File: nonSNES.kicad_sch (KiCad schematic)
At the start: 311 parts, among them J1 Jack-DC, P1 CASSETTE, P2 Conn_2Rows-11Pins, P3 Conn_01x02_Pin, Q10 C2412K, Q11 C2412K, Q12 C2412K, Q13 C2412K, Q14 C2412K, Q15 C2412K, Q16 C2412K, Q17 C2412K, Q18 C2412K, Q3 C2412K, Q4 C2412K, Q5 C2412K, Q6 C2412K, Q7 C2412K, Q8 C2412K, Q9 C2412K, SW1 RESET SW, T1 L_Coupled, U1 CPU, U10 LM324, U12 L7805, U13 S-SMP, U14 S-DSP, U15 MS62256CL-10FC, U16 MS62256CL-10FC, U17 uPD6376, U18 S-CLK, U2 PPU1, U3 PPU2, U4 MS62256CL-10FC, U5 MS62256CL-10FC, U6 WRAM, U7 S-ENC, U8 CIC, X1 17.734MHz, X2 24.576MHz

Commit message: fix errors
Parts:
- renumbered C20 to C12
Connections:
- net /IRQ: now also P5.26 (~{IRQ}), TP21.1
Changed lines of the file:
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@@
     )
   )
-  (global_label "{slash}IRQ" (shape input) (at 159.385 311.15 0) (fields_autoplaced)
+  (global_label "{slash}IRQ" (shape input) (at 158.75 311.15 0) (fields_autoplaced)
     (effects (font (size 1.27 1.27)) (justify left))
-    (property "Intersheetrefs" "${INTERSHEET_REFS}" (at 166.906 311.15 0)
+    (property "Intersheetrefs" "${INTERSHEET_REFS}" (at 166.271 311.15 0)
       (effects (font (size 1.27 1.27)) (justify left) hide)
     )
@@
   (symbol (lib_id "Device:C") (at 516.255 149.225 0) (unit 1)
     (in_bom yes) (on_board yes) (dnp no)
-    (property "Reference" "C20" (at 518.795 147.955 0)
+    (property "Reference" "C12" (at 518.795 147.955 0)
       (effects (font (size 1.27 1.27)) (justify left))
     )
@@
       (project "nonSNES"
         (path "/d1480d56-b791-43e1-bd4c-b0c74bb0533d"
-          (reference "C20") (unit 1)
+          (reference "C12") (unit 1)
         )
       )

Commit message: flip around most of the silkscreen on the bottom
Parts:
- renumbered C5 to C2, C2 to C5, C96 to C69, C69 to C96
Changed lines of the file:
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@@
   (symbol (lib_id "Device:C") (at 170.815 402.59 0) (mirror y) (unit 1)
     (in_bom no) (on_board yes) (dnp yes)
-    (property "Reference" "C96" (at 163.83 402.59 90)
+    (property "Reference" "C69" (at 163.83 402.59 90)
       (effects (font (size 1.27 1.27)))
     )
@@
       (project "nonSNES"
         (path "/d1480d56-b791-43e1-bd4c-b0c74bb0533d"
-          (reference "C96") (unit 1)
+          (reference "C69") (unit 1)
         )
       )
@@
   (symbol (lib_id "Device:C") (at 351.155 35.56 180) (unit 1)
     (in_bom yes) (on_board yes) (dnp no) (fields_autoplaced)
-    (property "Reference" "C69" (at 354.33 34.29 0)
+    (property "Reference" "C96" (at 354.33 34.29 0)
       (effects (font (size 1.27 1.27)) (justify right))
     )
@@
       (project "nonSNES"
         (path "/d1480d56-b791-43e1-bd4c-b0c74bb0533d"
-          (reference "C69") (unit 1)
+          (reference "C96") (unit 1)
         )
       )
@@
   (symbol (lib_id "Device:C") (at 131.445 387.985 90) (mirror x) (unit 1)
     (in_bom no) (on_board yes) (dnp yes)
-    (property "Reference" "C2" (at 131.445 394.97 90)
+    (property "Reference" "C5" (at 131.445 394.97 90)
       (effects (font (size 1.27 1.27)))
     )
@@
       (project "nonSNES"
         (path "/d1480d56-b791-43e1-bd4c-b0c74bb0533d"
-          (reference "C2") (unit 1)
+          (reference "C5") (unit 1)
         )
       )
@@
   (symbol (lib_id "Device:C") (at 131.445 370.84 90) (unit 1)
     (in_bom yes) (on_board yes) (dnp no) (fields_autoplaced)
-    (property "Reference" "C5" (at 131.445 363.22 90)
+    (property "Reference" "C2" (at 131.445 363.22 90)
       (effects (font (size 1.27 1.27)))
     )
@@
       (project "nonSNES"
         (path "/d1480d56-b791-43e1-bd4c-b0c74bb0533d"
-          (reference "C5") (unit 1)
+          (reference "C2") (unit 1)
         )
       )

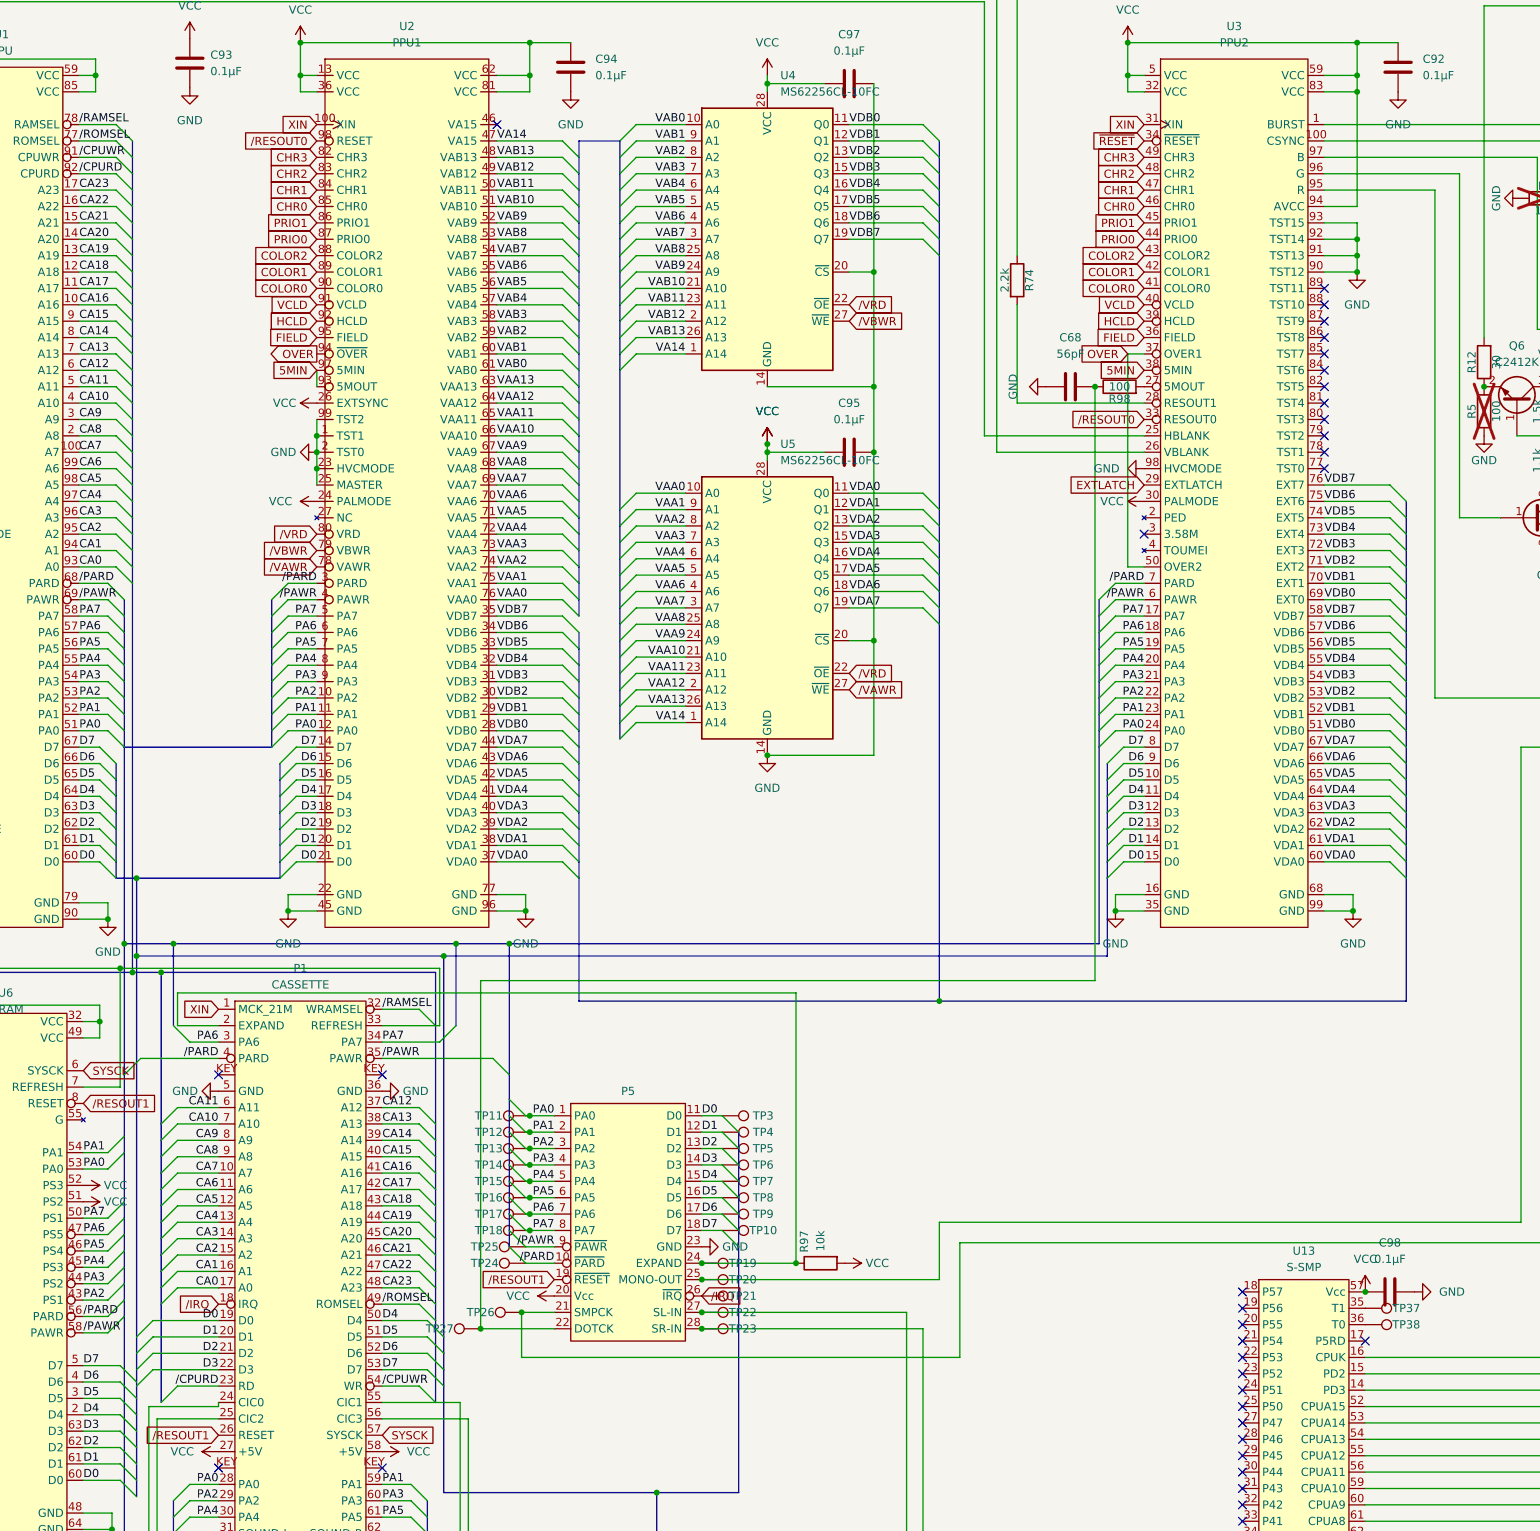
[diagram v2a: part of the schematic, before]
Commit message: add testpoints
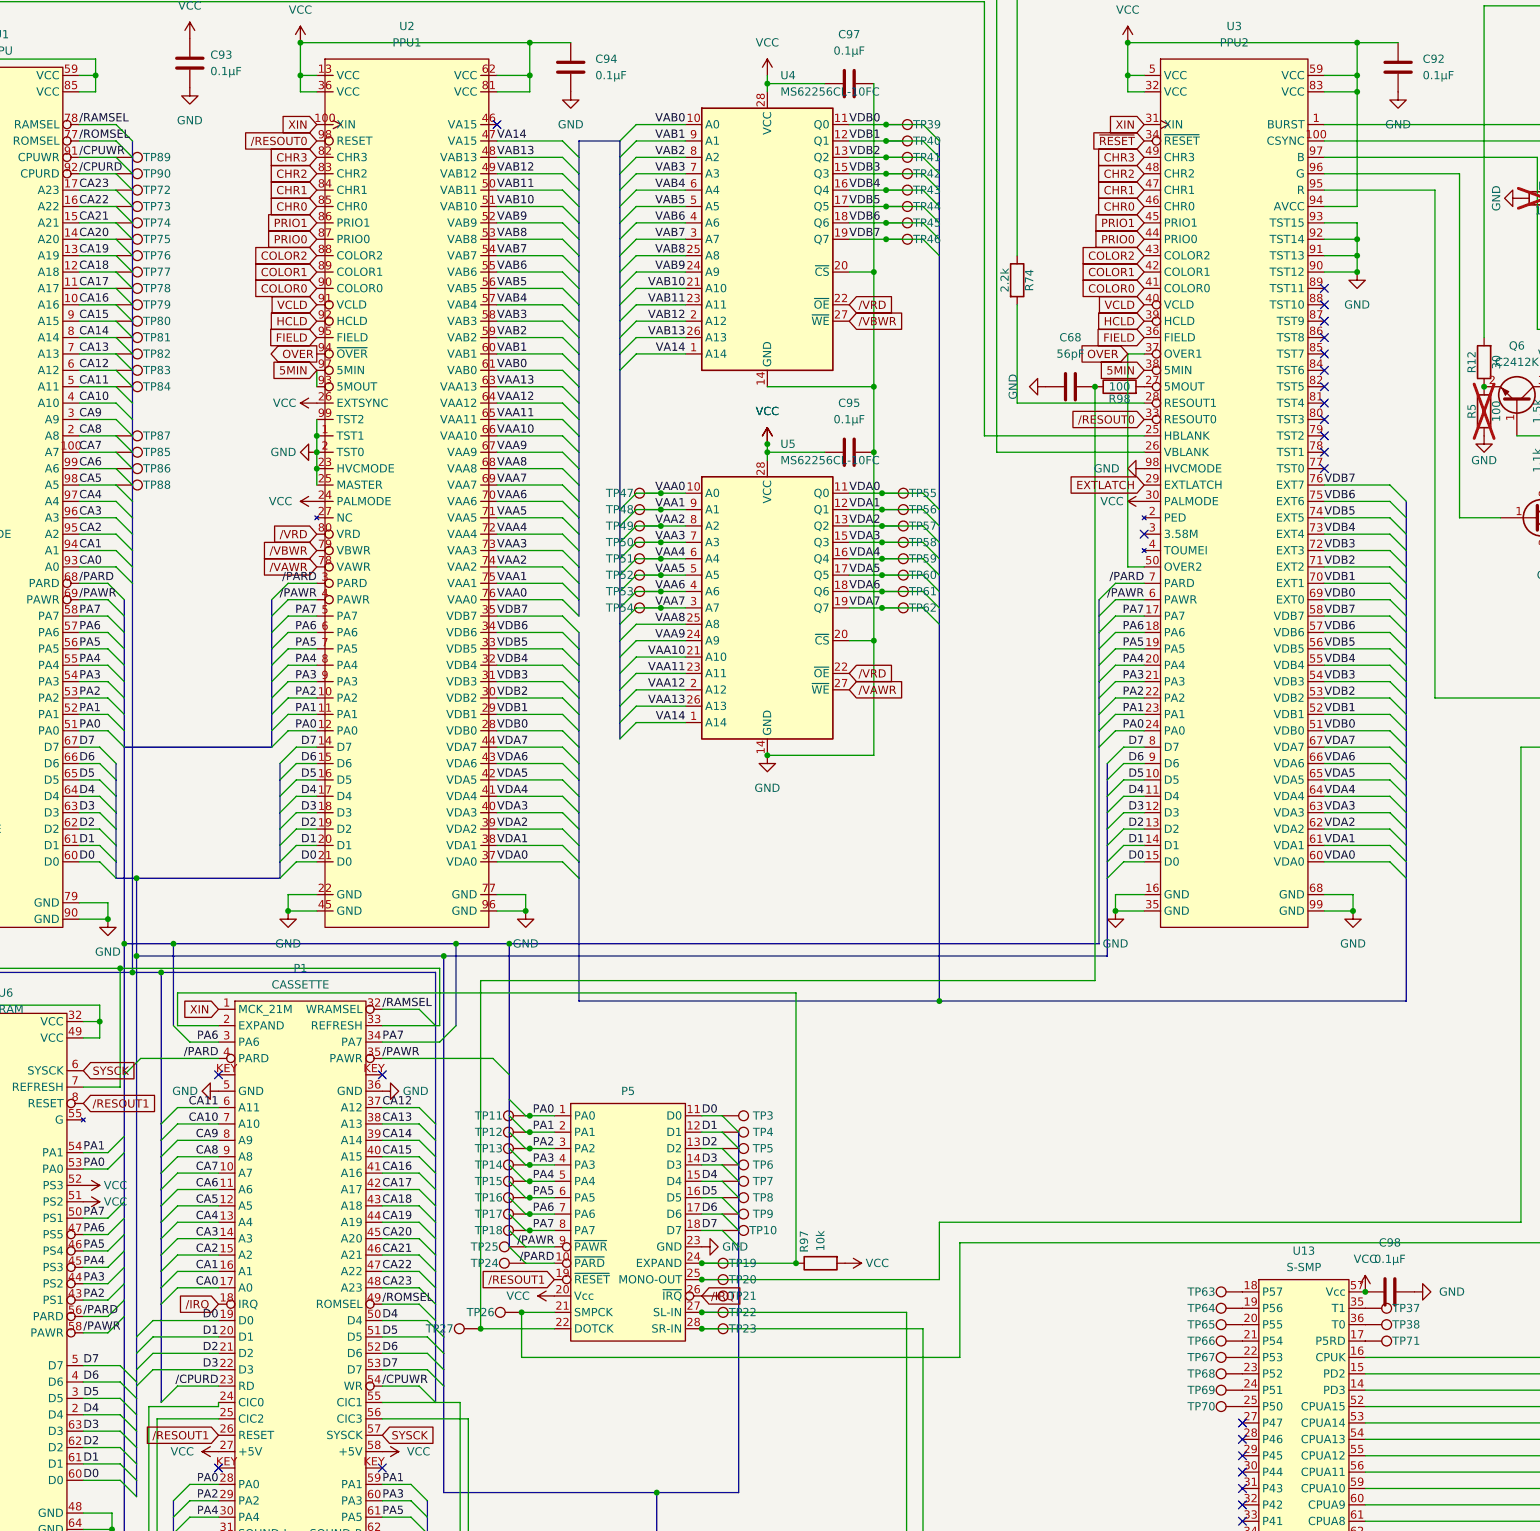
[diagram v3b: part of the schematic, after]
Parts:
- added TP39, TP40, TP41, TP42, TP43, TP44, TP45, TP46, TP47, TP48, TP49, TP50, TP51, TP52, TP53, TP54, TP55, TP56, TP57, TP58, TP59, TP60, TP61, TP62, TP63, TP64, TP65, TP66, TP67, TP68, TP69, TP70, TP71, TP72, TP73, TP74, TP75, TP76, TP77, TP78, TP79, TP80, TP81, TP82, TP83, TP84, TP85, TP86, TP87, TP88, TP89, TP90: TestPoint, TestPoint:TestPoint_Pad_D1.0mm, symbol Connector:TestPoint
- Q18: footprint Package_TO_SOT_SMD:SOT-23 -> Package_TO_SOT_SMD:SC-59
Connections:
- net CA11: now also TP84.1
- net CA12: now also TP83.1
- net CA13: now also TP82.1
- net CA14: now also TP81.1
- net CA15: now also TP80.1
- net CA16: now also TP79.1
- net CA17: now also TP78.1
- net CA18: now also TP77.1
- net CA19: now also TP76.1
- net CA20: now also TP75.1
- net CA21: now also TP74.1
- net CA22: now also TP73.1
- net CA23: now also TP72.1
- net CA5: now also TP88.1
- net CA6: now also TP86.1
- net CA7: now also TP85.1
- net CA8: now also TP87.1
- net VAA0: now also TP47.1
- net VAA1: now also TP48.1
- net VAA2: now also TP49.1
- net VAA3: now also TP50.1
- net VAA4: now also TP51.1
- net VAA5: now also TP52.1
- net VAA6: now also TP53.1
- net VAA7: now also TP54.1
- net VDA0: now also TP55.1
- net VDA1: now also TP56.1
- net VDA2: now also TP57.1
- net VDA3: now also TP58.1
- net VDA4: now also TP59.1
- net VDA5: now also TP60.1
- net VDA6: now also TP61.1
- net VDA7: now also TP62.1
- net VDB0: now also TP39.1
- net VDB1: now also TP40.1
- net VDB2: now also TP41.1
- net VDB3: now also TP42.1
- net VDB4: now also TP43.1
- net VDB5: now also TP44.1
- net VDB6: now also TP45.1
- net VDB7: now also TP46.1
- net /CPURD: now also TP90.1
- net /CPUWR: now also TP89.1
- net at U13.17 (P5RD): now also TP71.1
- net at U13.18 (P57): now also TP63.1
- net at U13.19 (P56): now also TP64.1
- net at U13.20 (P55): now also TP65.1
- net at U13.21 (P54): now also TP66.1
- net at U13.22 (P53): now also TP67.1
- net at U13.23 (P52): now also TP68.1
- net at U13.24 (P51): now also TP69.1
- net at U13.25 (P50): now also TP70.1
- no-connect marks 75 -> 66

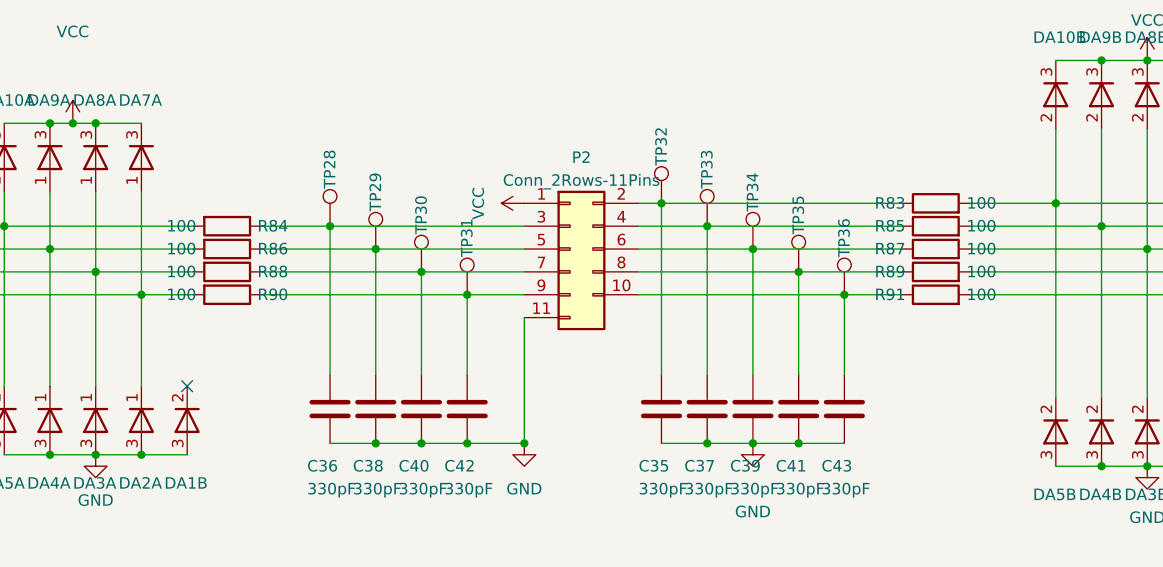
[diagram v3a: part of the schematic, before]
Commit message: these resistors are 10 ohms not 100
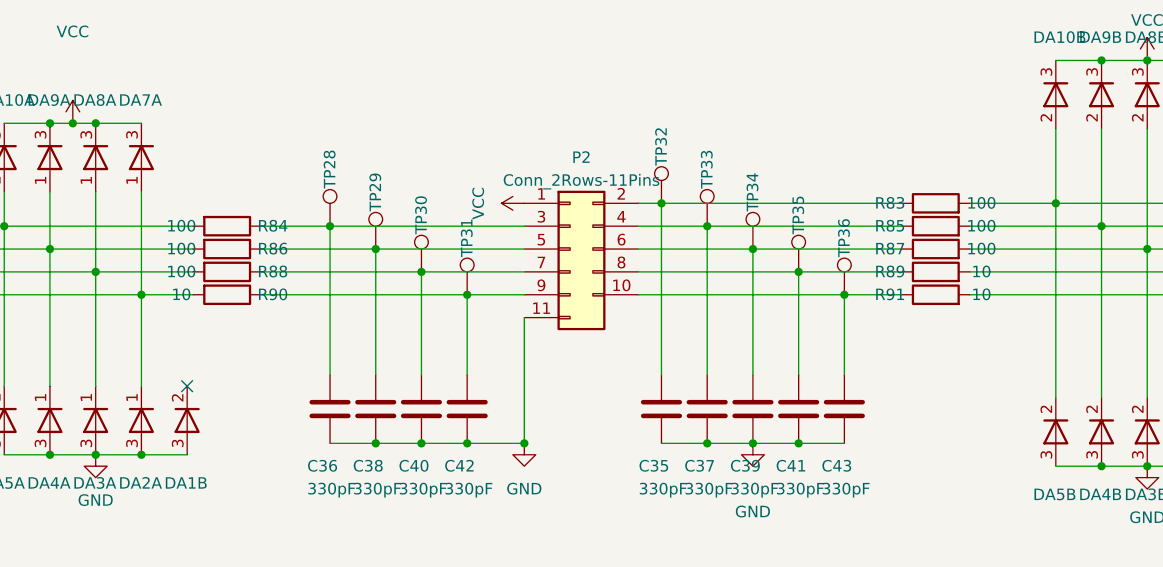
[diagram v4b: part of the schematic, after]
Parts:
- R89, R90, R91: value 100 -> 10
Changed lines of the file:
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@@
       (effects (font (size 1.27 1.27)))
     )
-    (property "Value" "100" (at 44.45 59.69 90)
+    (property "Value" "10" (at 44.45 59.69 90)
       (effects (font (size 1.27 1.27)))
     )
@@
       (effects (font (size 1.27 1.27)))
     )
-    (property "Value" "100" (at 133.35 57.15 90)
+    (property "Value" "10" (at 133.35 57.15 90)
       (effects (font (size 1.27 1.27)))
     )
@@
       (effects (font (size 1.27 1.27)))
     )
-    (property "Value" "100" (at 133.35 59.69 90)
+    (property "Value" "10" (at 133.35 59.69 90)
       (effects (font (size 1.27 1.27)))
     )
